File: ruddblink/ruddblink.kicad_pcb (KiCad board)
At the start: 2 copper layers, 40.6 x 48.5 mm, 30 parts, among them Q1 IRFML8244, SW1 JS202011JCQN, SW2 PTS526 SK15 SMTR2 LFS, U1 ATtiny85-20SU, U2 74HC595

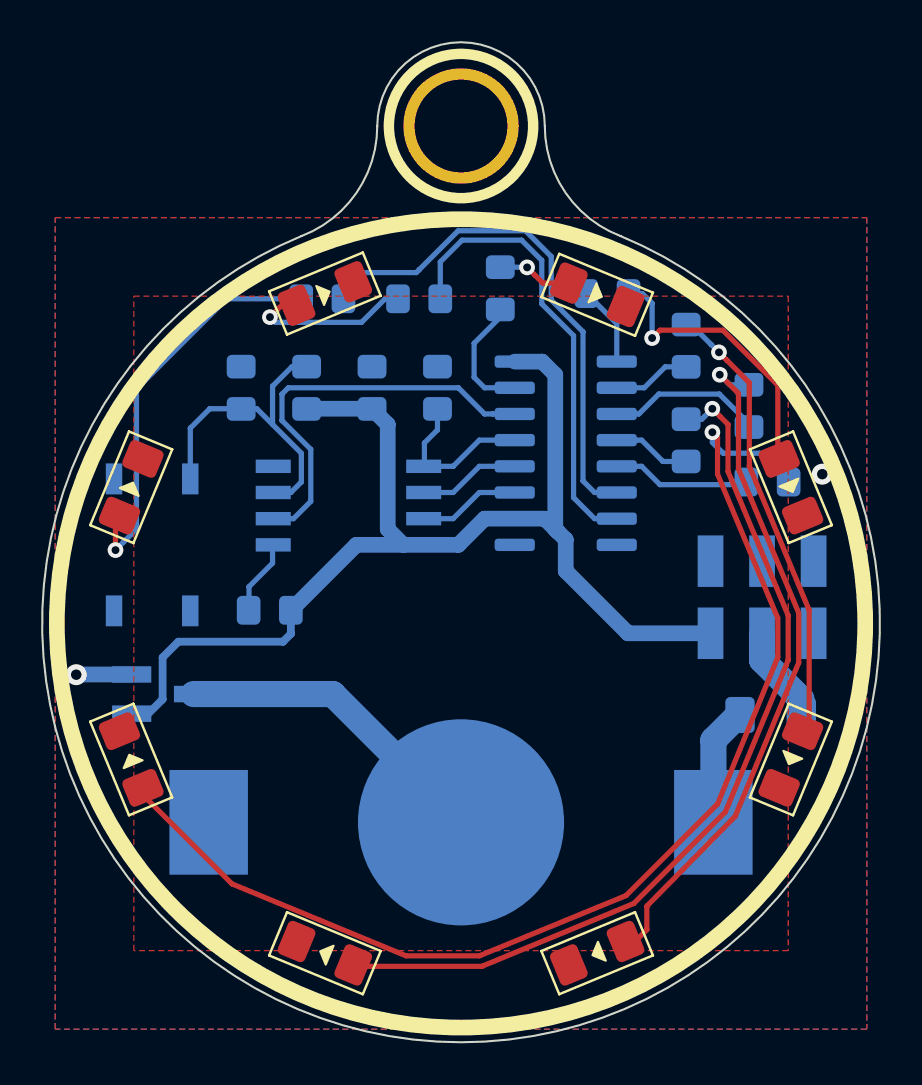
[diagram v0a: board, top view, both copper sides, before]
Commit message: Vanity edits
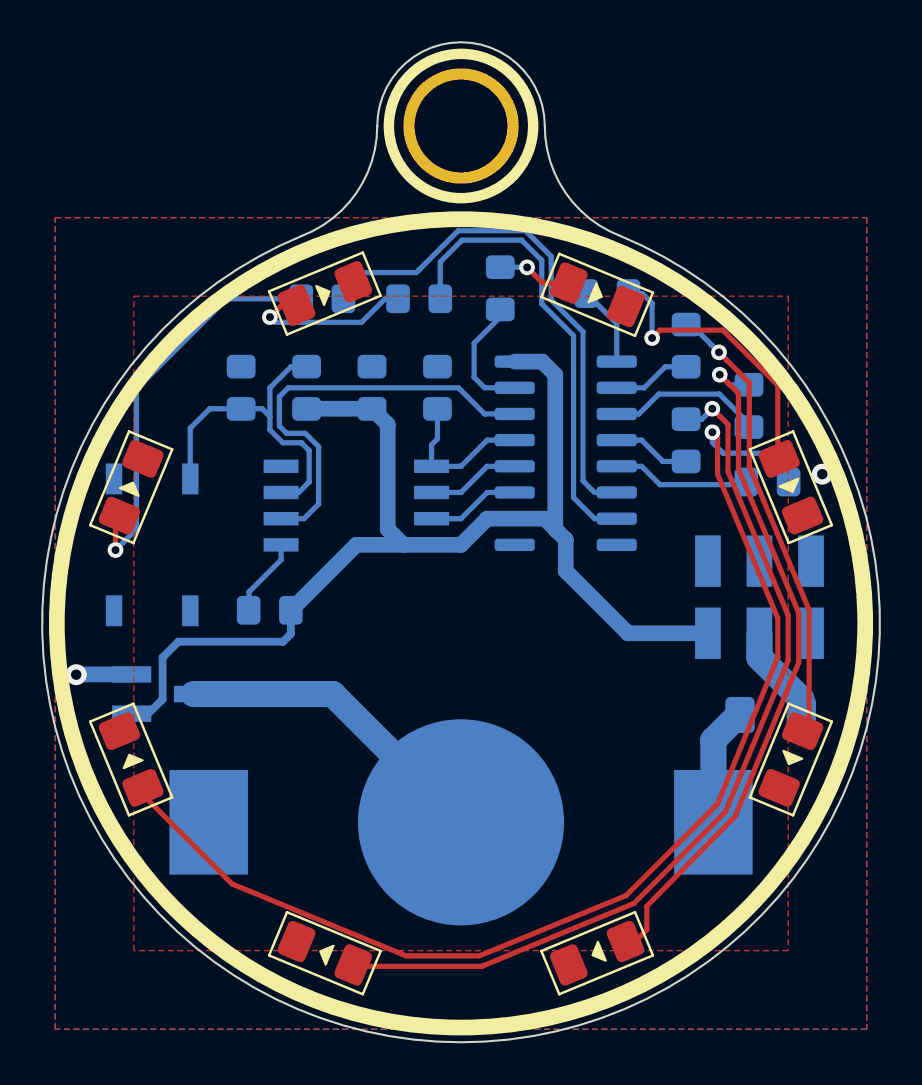
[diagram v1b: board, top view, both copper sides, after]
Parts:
- moved U1 0.38 mm to (137.2, 108.6)
- moved SW1 0.13 mm to (156.7, 113.0)
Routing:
- net /SER: track 20.2 -> 20.8 mm
